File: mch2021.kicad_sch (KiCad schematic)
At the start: 58 parts, among them J1 AudioJack3, J10 CONN-3, J12 Hook 1, J13 Hook 2, J2 USB_C_Receptacle_USB2.0, J3 QWIIC_CONNECTORJS-1MM, J4 PMOD, J6 QWIIC_CONNECTORJS-1MM, J9 CONN-7, U1 PCM5100, X1 Simple_Addon_v2

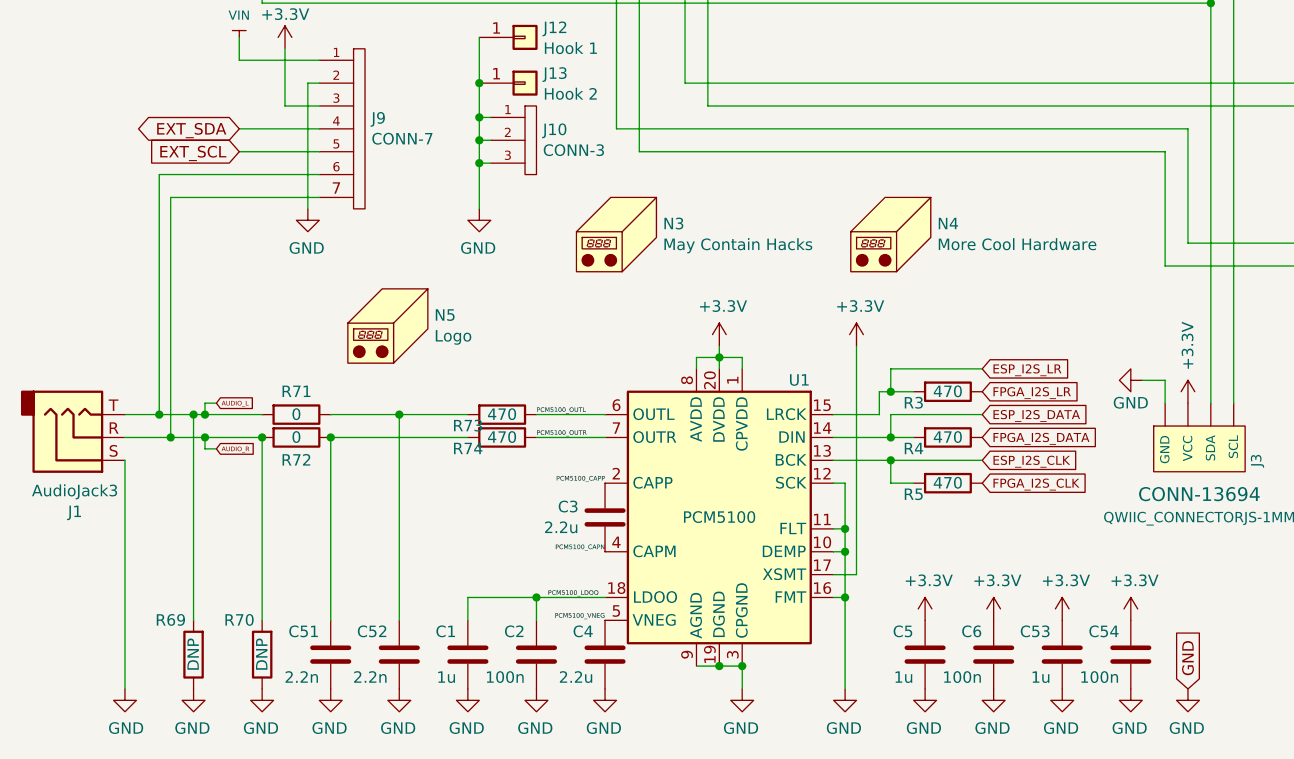
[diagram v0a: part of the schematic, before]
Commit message: Added audio amplifier TDA2822
Added an audio sheet, moved all the audio stuff there
Implemented TDA 2822 amplifier
Component choice and tuning need doing, putting a 100uF to 470uF electrolytic caps for DC bypass would be expensive
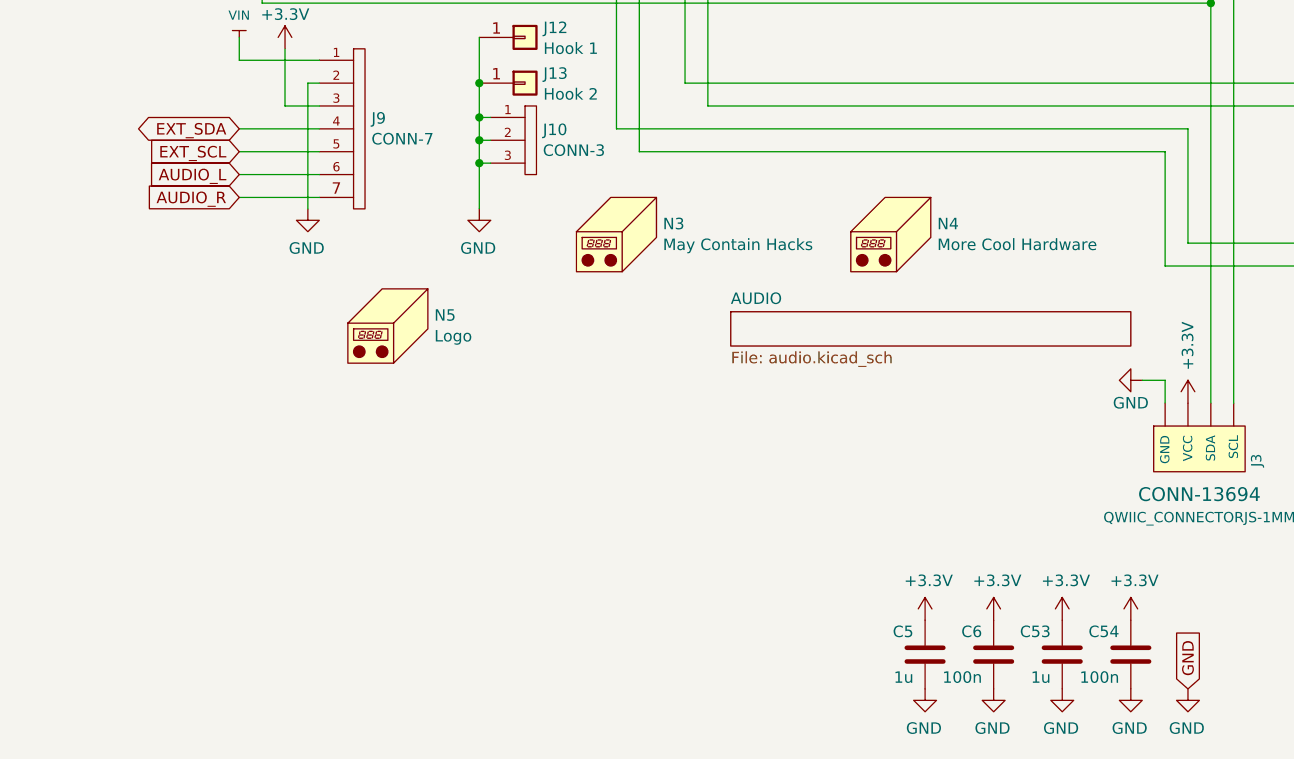
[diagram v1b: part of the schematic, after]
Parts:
- removed C1: 1u, Capacitor_SMD:C_0402_1005Metric, symbol mch2021-rescue:C-Device
- removed C2: 100n, Capacitor_SMD:C_0402_1005Metric, symbol mch2021-rescue:C-Device
- removed C3, C4: 2.2u, Capacitor_SMD:C_0402_1005Metric, symbol mch2021-rescue:C-Device
- removed C51, C52: 2.2n, Capacitor_SMD:C_0402_1005Metric, symbol mch2021-rescue:C-Device
- removed J1: AudioJack3, custom:Boom-audiojack-PJ-320B, symbol mch2021-rescue:AudioJack3-Connector
- removed R3, R4, R5, R73, R74: 470, Resistor_SMD:R_0402_1005Metric, symbol mch2021-rescue:R-Device
- removed R69, R70: DNP, Resistor_SMD:R_0402_1005Metric, symbol mch2021-rescue:R-Device
- removed R71, R72: 0, Resistor_SMD:R_0402_1005Metric, symbol mch2021-rescue:R-Device
- removed U1: PCM5100, Package_SO:TSSOP-20_4.4x6.5mm_P0.65mm, symbol mch2021-rescue:PCM5100-Audio
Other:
- added sheet AUDIO (audio.kicad_sch)
